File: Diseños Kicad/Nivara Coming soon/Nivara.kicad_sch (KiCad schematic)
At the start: 11 parts, among them J1 Screw_Terminal_01x02, J12 Screw_Terminal_01x04, J13 Screw_Terminal_01x02, J14 Screw_Terminal_01x06, J2 Screw_Terminal_01x04, J3 Screw_Terminal_01x02, J4 Screw_Terminal_01x02, J5 Screw_Terminal_01x03, J6 Screw_Terminal_01x02, J9 Screw_Terminal_01x03

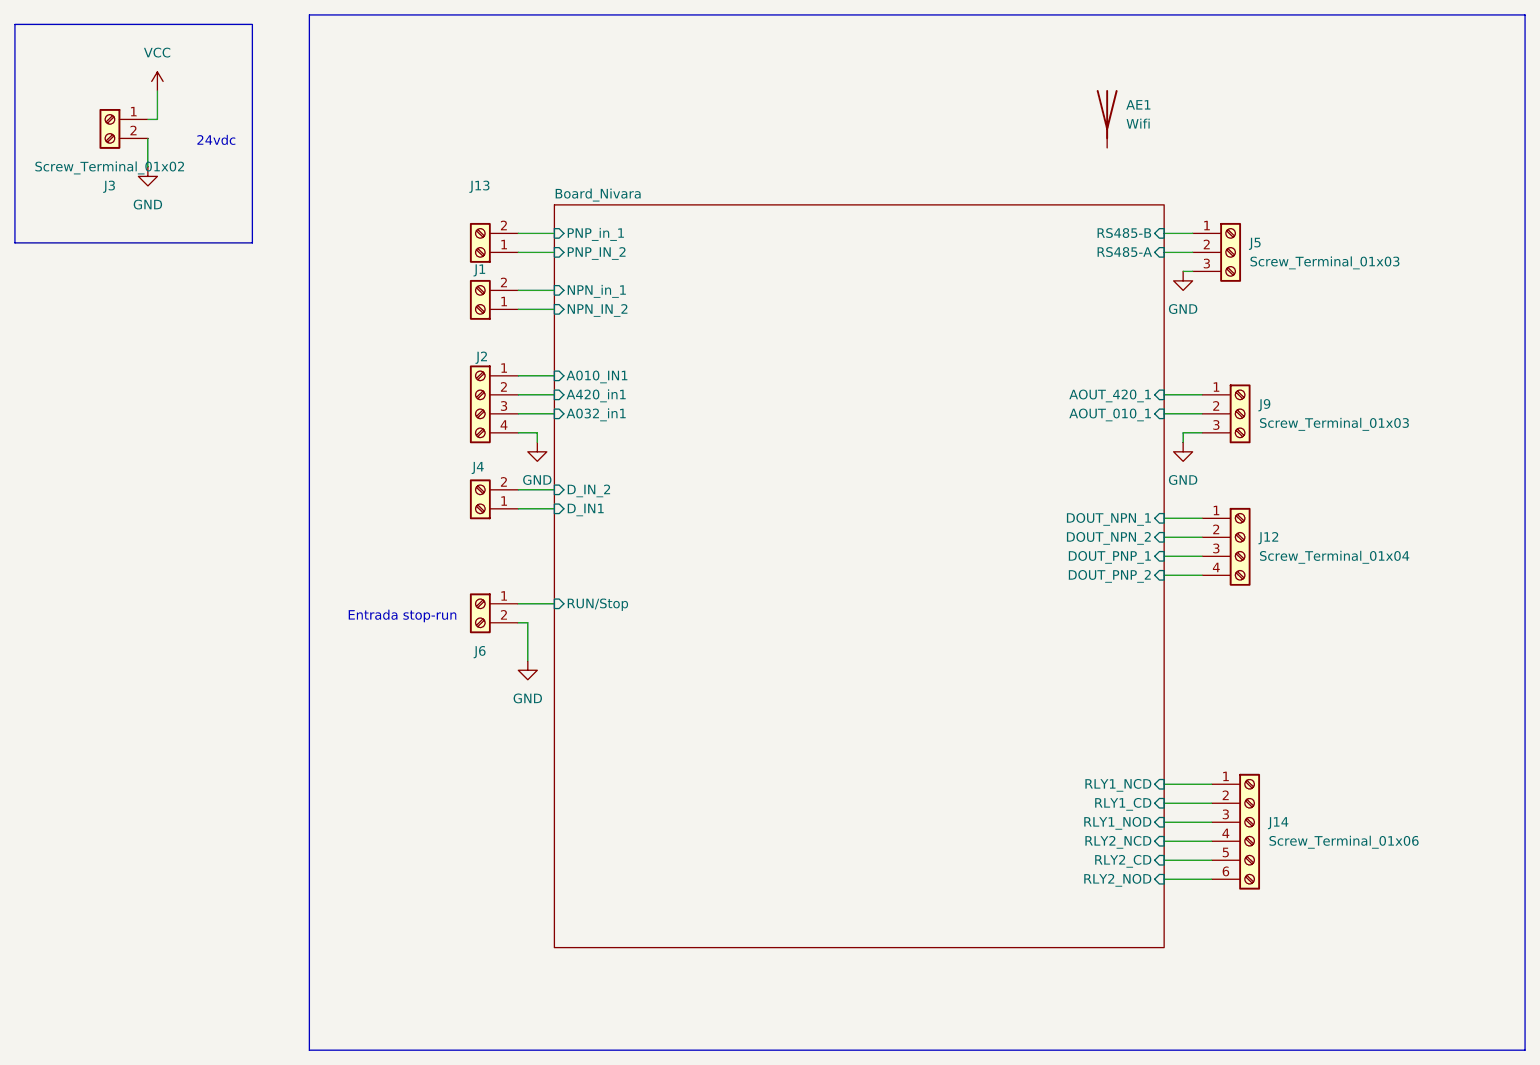
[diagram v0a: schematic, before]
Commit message: UPDATE TAREA
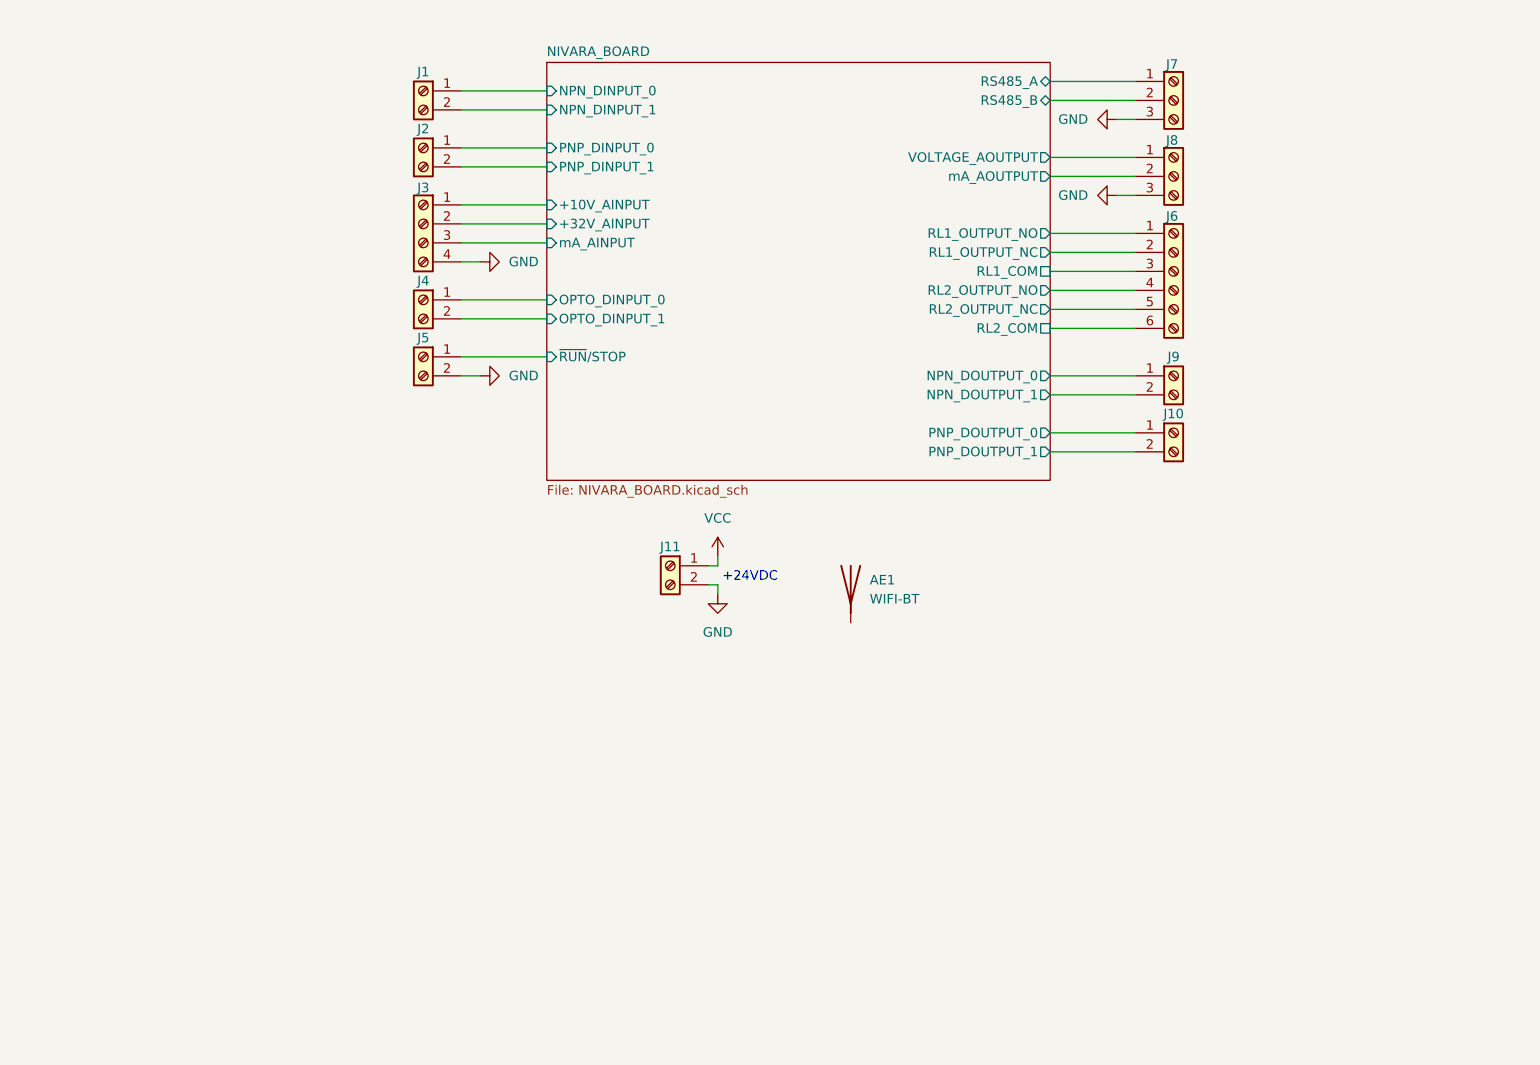
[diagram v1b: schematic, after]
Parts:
- removed J12, J2: Screw_Terminal_01x04, TerminalBlock_Phoenix:TerminalBlock_Phoenix_PT-1,5-4-5.0-H_1x04_P5.00mm_Horizontal, symbol Connector:Screw_Terminal_01x04
- removed J13, J3, J6: Screw_Terminal_01x02, TerminalBlock_Phoenix:TerminalBlock_Phoenix_PT-1,5-2-5.0-H_1x02_P5.00mm_Horizontal, symbol Connector:Screw_Terminal_01x02
- removed J14: Screw_Terminal_01x06, TerminalBlock_Phoenix:TerminalBlock_Phoenix_PT-1,5-6-5.0-H_1x06_P5.00mm_Horizontal, symbol Connector:Screw_Terminal_01x06
- removed J5, J9: Screw_Terminal_01x03, TerminalBlock_Phoenix:TerminalBlock_Phoenix_PT-1,5-3-3.5-H_1x03_P3.50mm_Horizontal, symbol Connector:Screw_Terminal_01x03
- added J10, J11, J2, J5, J9: Screw_Terminal_01x02, symbol Connector:Screw_Terminal_01x02
- added J3: Screw_Terminal_01x04, symbol Connector:Screw_Terminal_01x04
- added J6: Screw_Terminal_01x06, symbol Connector:Screw_Terminal_01x06
- added J7, J8: Screw_Terminal_01x03, symbol Connector:Screw_Terminal_01x03
- AE1: value Wifi -> WIFI-BT
- J1, J4: footprint TerminalBlock_Phoenix:TerminalBlock_Phoenix_PT-1,5-2-5.0-H_1x02_P5.00mm_Horizontal -> (none)
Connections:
- net GND: now also J11.2 (Pin_2), J3.4 (Pin_4), J5.2 (Pin_2), J7.3 (Pin_3), J8.3 (Pin_3)
- net VCC: now also J11.1 (Pin_1)
- net Board_Nivara/D_IN1 renamed NIVARA_BOARD/OPTO_DINPUT_0
- net Board_Nivara/D_IN_2 renamed NIVARA_BOARD/OPTO_DINPUT_1
- net Board_Nivara/NPN_IN_2 renamed NIVARA_BOARD/NPN_DINPUT_0
- net Board_Nivara/NPN_in_1 renamed NIVARA_BOARD/NPN_DINPUT_1
- new net NIVARA_BOARD/+10V_AINPUT: J3.1 (Pin_1)
- new net NIVARA_BOARD/+32V_AINPUT: J3.2 (Pin_2)
- new net NIVARA_BOARD/NPN_DOUTPUT_0: J9.1 (Pin_1)
- new net NIVARA_BOARD/NPN_DOUTPUT_1: J9.2 (Pin_2)
- new net NIVARA_BOARD/PNP_DINPUT_0: J2.1 (Pin_1)
- new net NIVARA_BOARD/PNP_DINPUT_1: J2.2 (Pin_2)
- new net NIVARA_BOARD/PNP_DOUTPUT_0: J10.1 (Pin_1)
- new net NIVARA_BOARD/PNP_DOUTPUT_1: J10.2 (Pin_2)
- new net NIVARA_BOARD/RL1_COM: J6.3 (Pin_3)
- new net NIVARA_BOARD/RL1_OUTPUT_NC: J6.2 (Pin_2)
- new net NIVARA_BOARD/RL1_OUTPUT_NO: J6.1 (Pin_1)
- new net NIVARA_BOARD/RL2_COM: J6.6 (Pin_6)
- new net NIVARA_BOARD/RL2_OUTPUT_NC: J6.5 (Pin_5)
- new net NIVARA_BOARD/RL2_OUTPUT_NO: J6.4 (Pin_4)
- new net NIVARA_BOARD/RS485_A: J7.1 (Pin_1)
- new net NIVARA_BOARD/RS485_B: J7.2 (Pin_2)
- new net NIVARA_BOARD/VOLTAGE_AOUTPUT: J8.1 (Pin_1)
- new net NIVARA_BOARD/mA_AINPUT: J3.3 (Pin_3)
- new net NIVARA_BOARD/mA_AOUTPUT: J8.2 (Pin_2)
- new net NIVARA_BOARD/~{RUN}/STOP: J5.1 (Pin_1)
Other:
- removed sheet Board_Nivara
- added sheet NIVARA_BOARD (NIVARA_BOARD.kicad_sch)
- note added: "+24VDC"
- note removed: "24vdc"
- note removed: "Entrada stop-run"
- company: Electia_ITLA -> (none)
- title: ZorionX-Nivara -> (none)
